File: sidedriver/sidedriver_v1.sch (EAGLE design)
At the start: 28 parts, among them IC2 LD117AD2MTR, Q1 8MHz

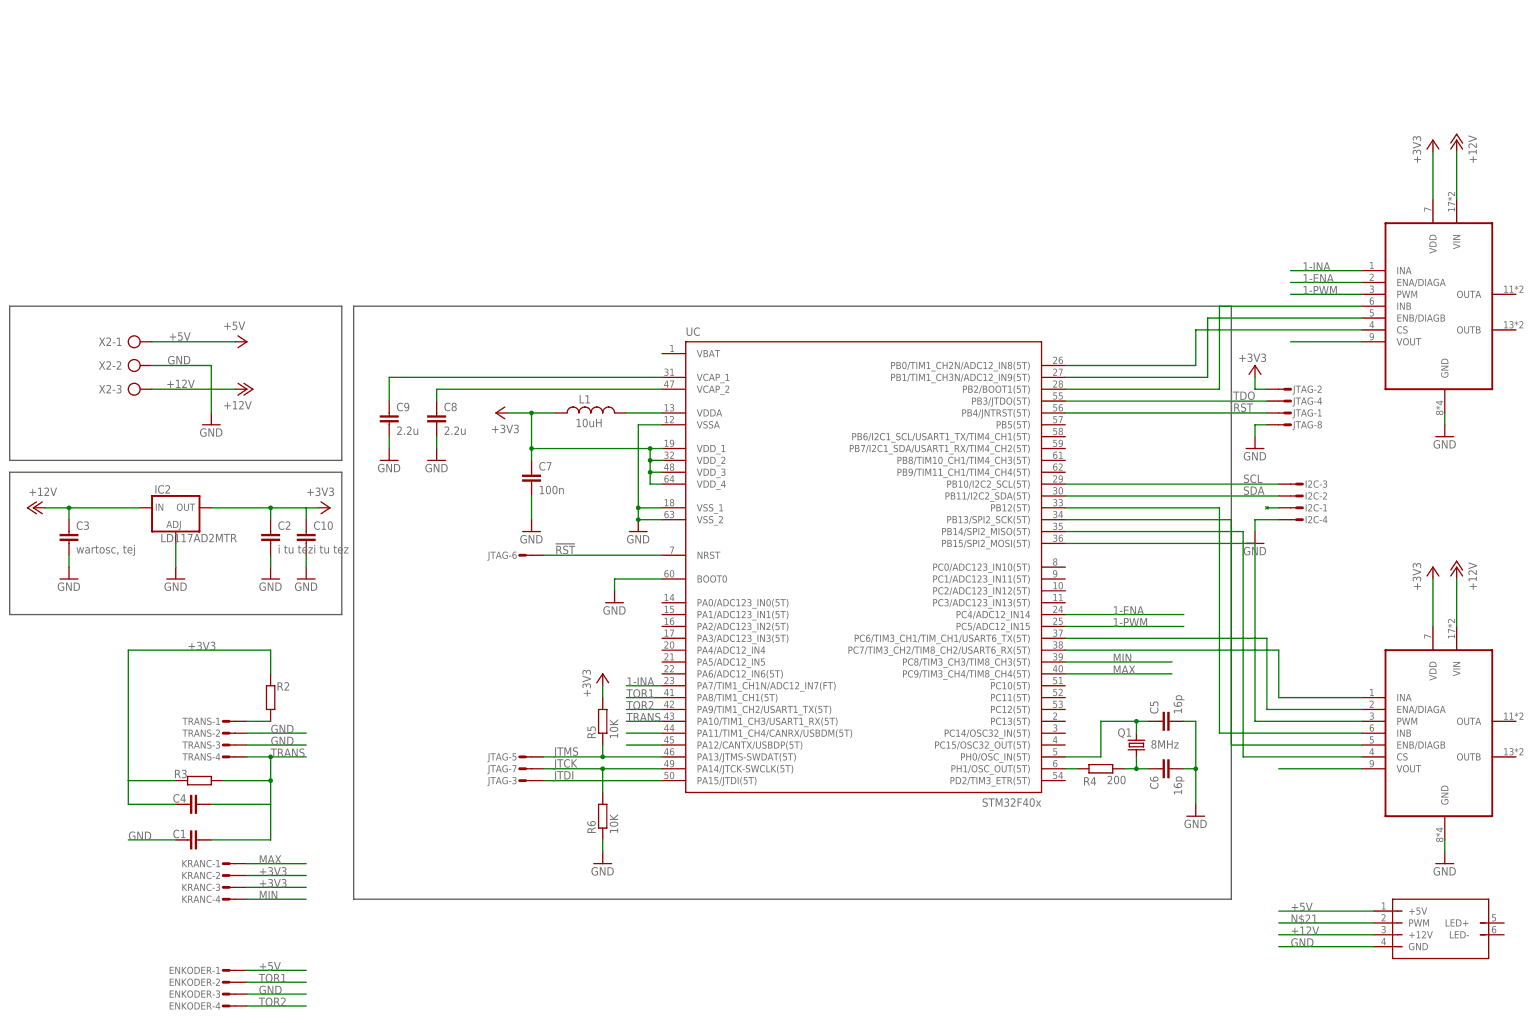
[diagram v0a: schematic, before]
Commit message: 03-12-13 20:52
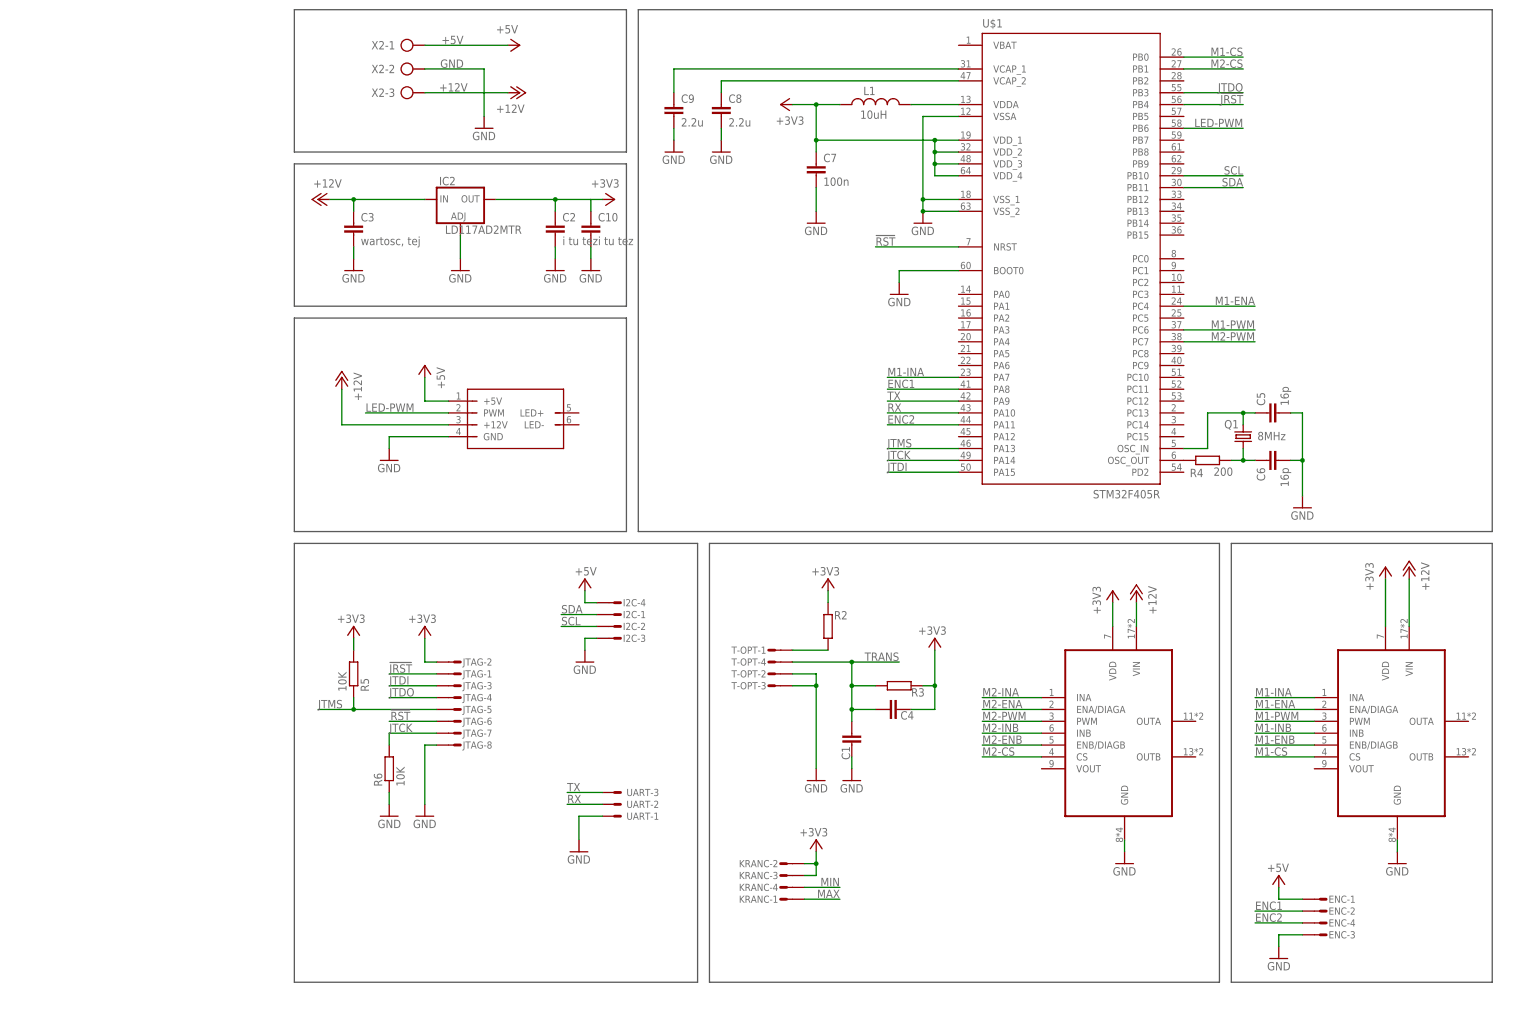
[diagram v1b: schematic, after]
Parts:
- removed ENKODER, TRANS: MICROMATCH-4, con-maritex:MICROMATCH-4
- removed UC: STM32F405RGT, stm32f4:STM32F405R
- added ENC, T-OPT: MICROMATCH-4, con-maritex:MICROMATCH-4
- added U$1: STM32F405R, stm32f4:STM32F405R
- added UART: C-GRID-03-70543, con-molex:C-GRID-03-70543
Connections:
- removed net 1-ENA: U$4.ENA/DIAGA, UC.PC4/ADC12_IN14
- removed net 1-INA: U$4.INA, UC.PA7/TIM1_CH1N/ADC12_IN7(FT)
- removed net 1-PWM: U$4.PWM, UC.PC5/ADC12_IN15
- removed net N$10: U$4.ENB/DIAGB, UC.PB1/TIM1_CH3N/ADC12_IN9(5T)
- removed net N$11: U$4.CS, UC.PB0/TIM1_CH2N/ADC12_IN8(5T)
- removed net N$12: U$4.VOUT
- removed net N$13: U$3.INB, UC.PB12(5T)
- removed net N$15: U$3.PWM, UC.PB15/SPI2_MOSI(5T)
- removed net N$17: U$3.ENB/DIAGB, UC.PB13/SPI2_SCK(5T)
- removed net N$18: U$3.CS, UC.PB14/SPI2_MISO(5T)
- removed net N$19: U$3.VOUT
- removed net N$21: U$2.PWM
- removed net N$25: I2C-1.S
- removed net N$38: U$3.ENA/DIAGA, UC.PC6/TIM3_CH1/TIM_CH1/USART6_TX(5T)
- removed net N$39: U$3.INA, UC.PC7/TIM3_CH2/TIM8_CH2/USART6_RX(5T)
- removed net N$6: U$4.INB, UC.PB2/BOOT1(5T)
- removed net N$7: UC.PA12/CANTX/USBDP(5T)
- removed net N$8: UC.PA11/TIM1_CH4/CANRX/USBDM(5T)
- removed net TOR1: ENKODER-2.S, UC.PA8/TIM1_CH1(5T)
- removed net TOR2: ENKODER-4.S, UC.PA9/TIM1_CH2/USART1_TX(5T)
- new net ENC1: ENC-2.S, U$1.PA8
- new net ENC2: ENC-4.S, U$1.PA11
- new net LED-PWM: U$1.PB6, U$2.PWM
- new net M1-CS: U$1.PB0, U$4.CS
- new net M1-ENA: U$1.PC4, U$4.ENA/DIAGA
- new net M1-ENB: U$4.ENB/DIAGB
- new net M1-INA: U$1.PA7, U$4.INA
- new net M1-INB: U$4.INB
- new net M1-PWM: U$1.PC6, U$4.PWM
- new net M2-CS: U$1.PB1, U$3.CS
- new net M2-ENA: U$3.ENA/DIAGA
- new net M2-ENB: U$3.ENB/DIAGB
- new net M2-INA: U$3.INA
- new net M2-INB: U$3.INB
- new net M2-PWM: U$1.PC7, U$3.PWM
- new net RX: U$1.PA10, UART-2.S
- new net TX: U$1.PA9, UART-3.S
- net !JRST: now also U$1.PB4; no longer UC.PB4/JNTRST(5T)
- net !RST: now also U$1.NRST; no longer UC.NRST
- net +3V3: now also U$1.VDD_1, U$1.VDD_2, U$1.VDD_3, U$1.VDD_4; no longer UC.VDD_1, UC.VDD_2, UC.VDD_3, UC.VDD_4
- net +5V: now also ENC-1.S, I2C-4.S; no longer ENKODER-1.S
- net GND: now also ENC-3.S, I2C-3.S, T-OPT-2.S, T-OPT-3.S, U$1.BOOT0, U$1.VSSA, U$1.VSS_1, U$1.VSS_2, UART-1.S; no longer ENKODER-3.S, I2C-4.S, TRANS-2.S, TRANS-3.S, UC.BOOT0, UC.VSSA, UC.VSS_1, UC.VSS_2
- net JTCK: now also U$1.PA14; no longer UC.PA14/JTCK-SWCLK(5T)
- net JTDI: now also U$1.PA15; no longer UC.PA15/JTDI(5T)
- net JTDO: now also U$1.PB3; no longer UC.PB3/JTDO(5T)
- net JTMS: now also U$1.PA13; no longer UC.PA13/JTMS-SWDAT(5T)
- net MAX: no longer UC.PC9/TIM3_CH4/TIM8_CH4(5T)
- net MIN: no longer UC.PC8/TIM3_CH3/TIM8_CH3(5T)
- net N$1: now also T-OPT-1.S; no longer TRANS-1.S
- net N$20: now also U$1.VDDA; no longer UC.VDDA
- net N$22: now also U$1.OSC_OUT; no longer UC.PH1/OSC_OUT(5T)
- net N$23: now also U$1.VCAP_2; no longer UC.VCAP_2
- net N$24: now also U$1.VCAP_1; no longer UC.VCAP_1
- net N$5: now also U$1.OSC_IN; no longer UC.PH0/OSC_IN(5T)
- net SCL: now also I2C-2.S, U$1.PB10; no longer I2C-3.S, UC.PB10/I2C2_SCL(5T)
- net SDA: now also I2C-1.S, U$1.PB11; no longer I2C-2.S, UC.PB11/I2C2_SDA(5T)
- net TRANS: now also T-OPT-4.S; no longer TRANS-4.S, UC.PA10/TIM1_CH3/USART1_RX(5T)
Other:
- moved on the sheet: C1, C10, C2, C3, C4, C5, C6, C7, C8, C9, I2C-1, I2C-2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
